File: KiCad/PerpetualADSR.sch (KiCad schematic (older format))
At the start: 38 parts, among them J1 TEST_CONN, J2 GATE, J3 CLOCK, J4 PWR_Conn, J5 OUT, SW1 EXP/LIN, U1 ATmega328P-PU, U2 MCP4921, U3 MCP3208, Y1 16MHz

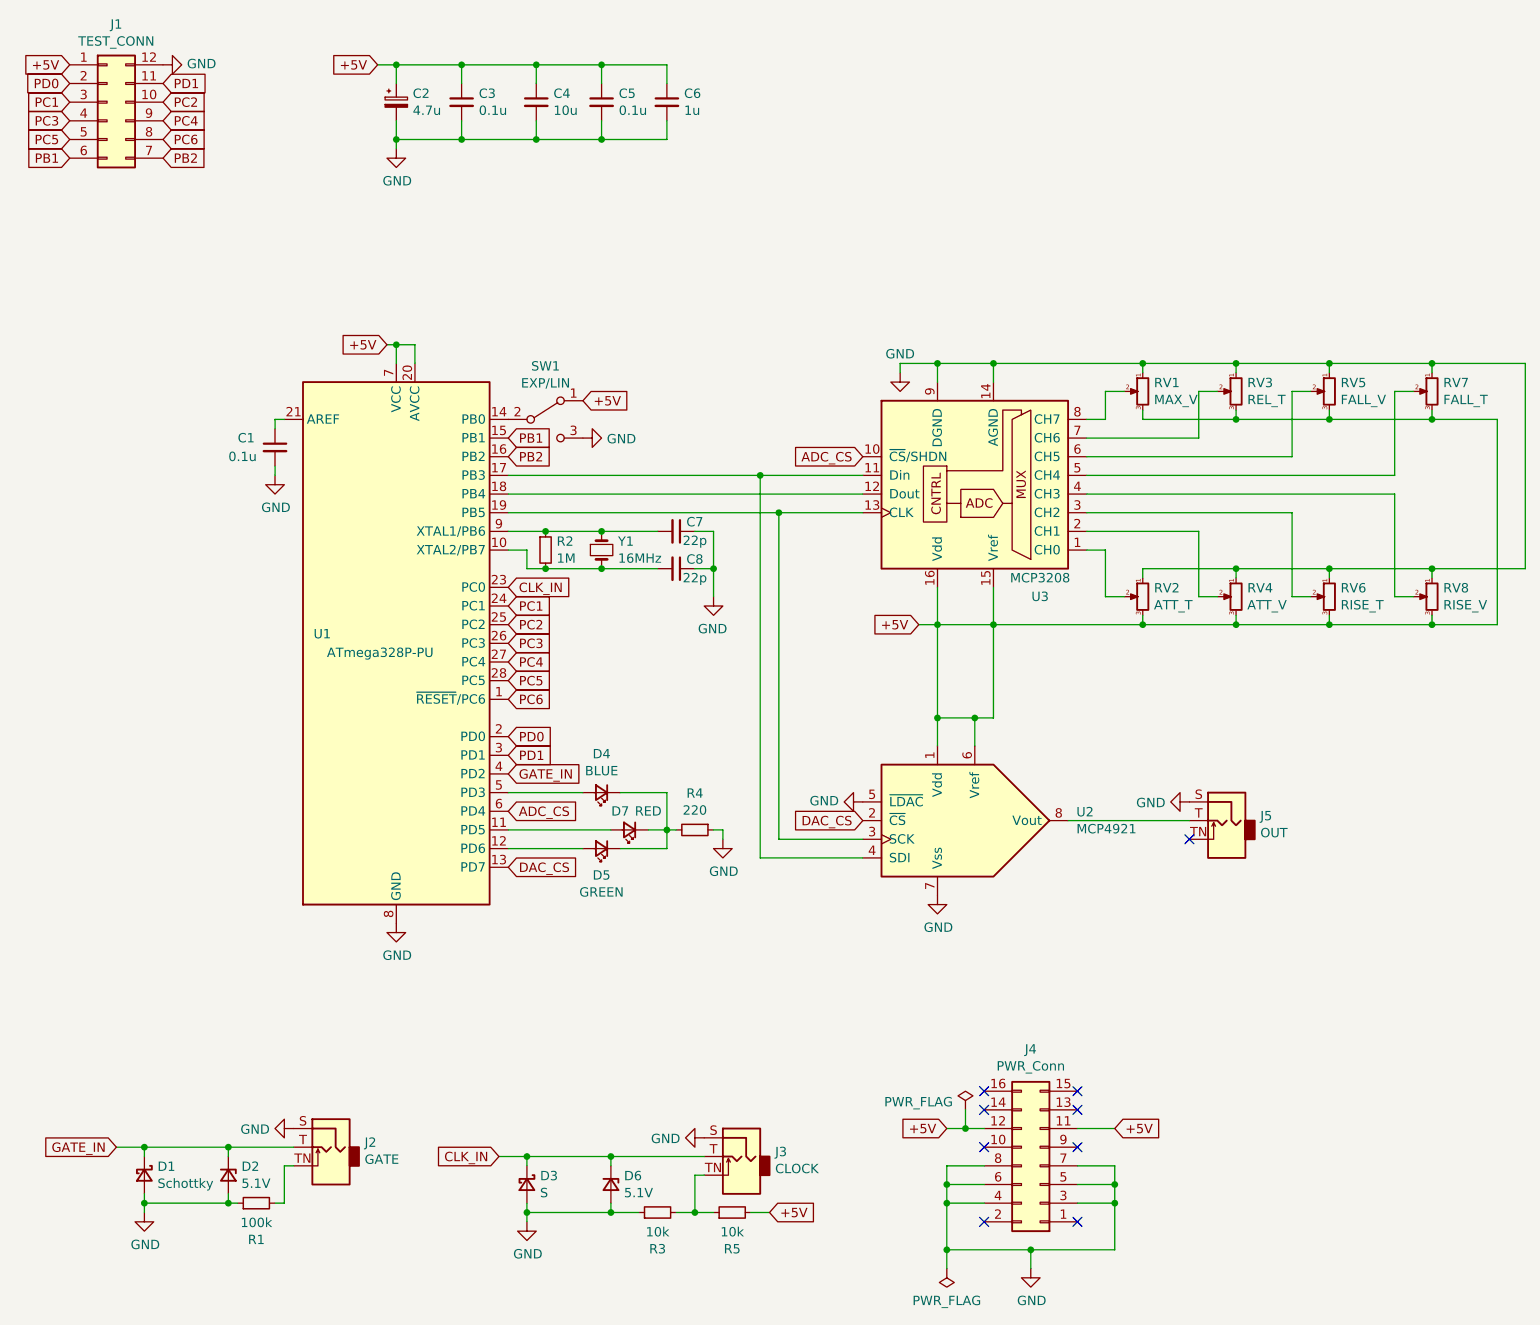
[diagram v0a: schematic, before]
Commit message: started PCB
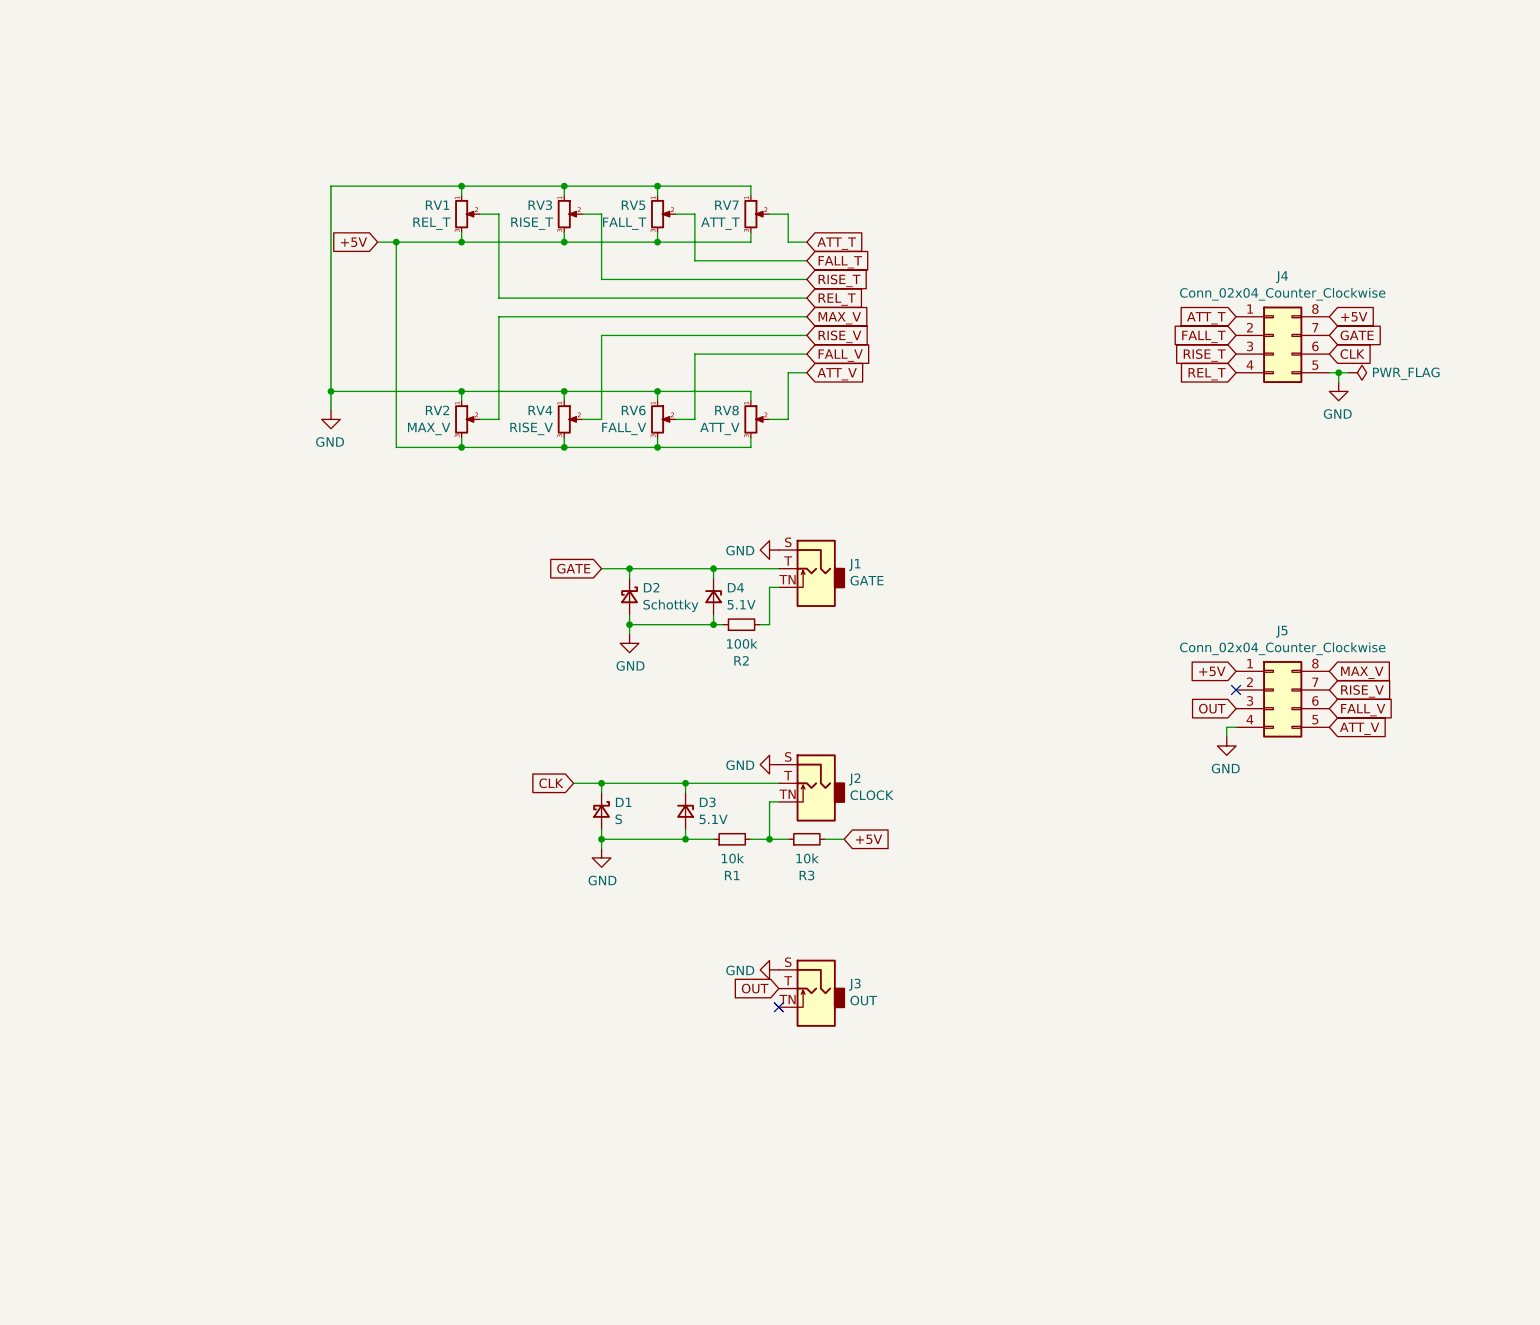
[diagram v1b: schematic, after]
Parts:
- removed C1, C3, C5: 0.1u, Capacitor_THT:C_Disc_D5.0mm_W2.5mm_P5.00mm, symbol Device:C_Small
- removed C2: 4.7u, Capacitor_THT:C_Disc_D5.0mm_W2.5mm_P2.50mm, symbol Device:CP_Small
- removed C4: 10u, Capacitor_THT:C_Disc_D5.0mm_W2.5mm_P5.00mm, symbol Device:C_Small
- removed C6: 1u, Capacitor_THT:C_Disc_D5.0mm_W2.5mm_P2.50mm, symbol Device:C_Small
- removed C7, C8: 22p, Capacitor_THT:C_Disc_D5.0mm_W2.5mm_P5.00mm, symbol Device:C_Small
- removed D4: BLUE, LED_THT:LED_D5.0mm, symbol Device:LED_Small
- removed D5: GREEN, LED_THT:LED_D5.0mm, symbol Device:LED_Small
- removed D7: RED, LED_THT:LED_D5.0mm, symbol Device:LED_Small
- removed J1: TEST_CONN, Connector_PinHeader_2.54mm:PinHeader_2x06_P2.54mm_Vertical, symbol Connector_Generic:Conn_02x06_Counter_Clockwise
- removed J4: PWR_Conn, Connector_IDC:IDC-Header_2x08_P2.54mm_Vertical, symbol Connector_Generic:Conn_02x08_Odd_Even
- removed R2: 1M, Resistor_THT:R_Axial_DIN0207_L6.3mm_D2.5mm_P7.62mm_Horizontal, symbol Device:R_Small
- removed R4: 220, Resistor_THT:R_Axial_DIN0207_L6.3mm_D2.5mm_P7.62mm_Horizontal, symbol Device:R_Small
- removed SW1: EXP/LIN, PerpetualADSR:SLIDE_SW_OS102011MS2QN1, symbol Switch:SW_SPDT
- removed U1: ATmega328P-PU, Package_DIP:DIP-28_W7.62mm, symbol MCU_Microchip_ATmega:ATmega328P-PU
- removed U2: MCP4921, Package_DIP:DIP-8_W7.62mm, symbol Analog_DAC:MCP4921
- removed U3: MCP3208, Package_DIP:DIP-16_W7.62mm, symbol Analog_ADC:MCP3208
- removed Y1: 16MHz, Crystal:Crystal_HC49-4H_Vertical, symbol Device:Crystal_Small
- added J4, J5: Conn_02x04_Counter_Clockwise, Connector_PinSocket_2.54mm:PinSocket_2x04_P2.54mm_Vertical, symbol Connector_Generic:Conn_02x04_Counter_Clockwise
- RV1: renamed from RV7; value FALL_T -> REL_T
- RV2: renamed from RV8; value RISE_V -> MAX_V
- RV3: renamed from RV5; value FALL_V -> RISE_T
- RV4: renamed from RV6; value RISE_T -> RISE_V
- RV5: renamed from RV3; value REL_T -> FALL_T
- RV6: renamed from RV4; value ATT_V -> FALL_V
- RV7: renamed from RV1; value MAX_V -> ATT_T
- RV8: renamed from RV2; value ATT_T -> ATT_V
- renumbered D3 to D1, D1 to D2, D6 to D3, D2 to D4, J2 to J1, J3 to J2, J5 to J3, R3 to R1, R1 to R2, R5 to R3
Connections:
- net +5V: now also J4.8 (Pin_8), J5.1 (Pin_1)
- net GND: now also J4.5 (Pin_5), J5.4 (Pin_4)
- net ATT_V: now reaches RV8.2
- net ATT_V: now also J5.5 (Pin_5)
- net FALL_V: now reaches RV6.2
- net FALL_V: now also J5.6 (Pin_6)
- net RISE_V: now reaches RV4.2
- net RISE_V: now also J5.7 (Pin_7)
- net MAX_V: now reaches RV2.2
- net MAX_V: now also J5.8 (Pin_8)
- net REL_T: now reaches RV1.2
- net REL_T: now also J4.4 (Pin_4)
- net RISE_T: now reaches RV3.2
- net RISE_T: now also J4.3 (Pin_3)
- net FALL_T: now reaches RV5.2
- net FALL_T: now also J4.2 (Pin_2)
- net ATT_T: now reaches RV7.2
- net ATT_T: now also J4.1 (Pin_1)
- net OUT: now reaches J3.T
- net OUT: now also J5.3 (Pin_3)
- net CLK_IN renamed CLK
- net CLK: now also J4.6 (Pin_6)
- net GATE_IN renamed GATE
- net GATE: now also J4.7 (Pin_7)
- no-connect marks 9 -> 2
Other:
- moved on the sheet: D1, D2, D3, D4, J1, J2, J3, R1, R2, R3, RV1, RV2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
